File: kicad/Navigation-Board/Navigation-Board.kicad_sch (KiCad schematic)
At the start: 179 parts, among them J25 2.8" TFT, J26 0.96" OLED, J27 Conn_01x02, J28 GME0831B, J31 Conn_01x04, SW10 SW_SPST, SW11 SW_SPST, SW12 SW_SPST, SW13 SW_SPST, SW14 SW_SPST, SW15 SW_SPST, SW16 SW_SPST, SW17 SW_SPST, SW18 SW_SPST, SW19 SW_SPST, SW2 SW_SPST, SW20 SW_SPST, SW21 SW_SPST, SW22 SW_SPST, SW23 SW_SPST, SW24 SW_SPST, SW25 SW_SPST, SW26 SW_SPST, SW27 SW_SPST, SW28 SW_SPST, SW29 SW_SPST, SW3 SW_SPST, SW30 SW_SPST, SW31 SW_SPST, SW32 SW_SPST, SW33 SW_SPST, SW34 SW_SPST, SW35 SW_SPST, SW36 SW_SPST, SW37 SW_SPST, SW38 SW_SPST, SW39 SW_SPST, SW4 SW_SPST, SW40 SW_SPST, SW41 SW_SPST, SW42 SW_SPST, SW43 SW_SPST, SW44 SW_SPST, SW45 SW_SPST, SW46 SW_SPST, SW47 SW_SPST, SW48 SW_SPST, SW49 SW_SPST, SW5 SW_SPST, SW50 SW_SPST, SW51 SW_SPST, SW52 SW_SPST, SW53 SW_SPST, SW54 SW_SPST, SW55 SW_SPST, SW56 SW_SPST, SW57 SW_SPST, SW58 SW_SPST, SW59 SW_SPST, SW6 SW_SPST, SW60 SW_SPST, SW61 SW_SPST, SW62 SW_SPST, SW63 SW_SPST, SW64 SW_SPST, SW65 SW_SPST, SW66 SW_SPST, SW67 SW_SPST, SW68 SW_SPST, SW69 SW_SPST, SW7 SW_SPST, SW70 SW_SPST, SW71 SW_SPST, SW72 SW_SPST, SW73 SW_SPST, SW74 SW_SPST, SW75 SW_SPST, SW76 SW_SPST, SW77 SW_SPST, SW78 SW_SPST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

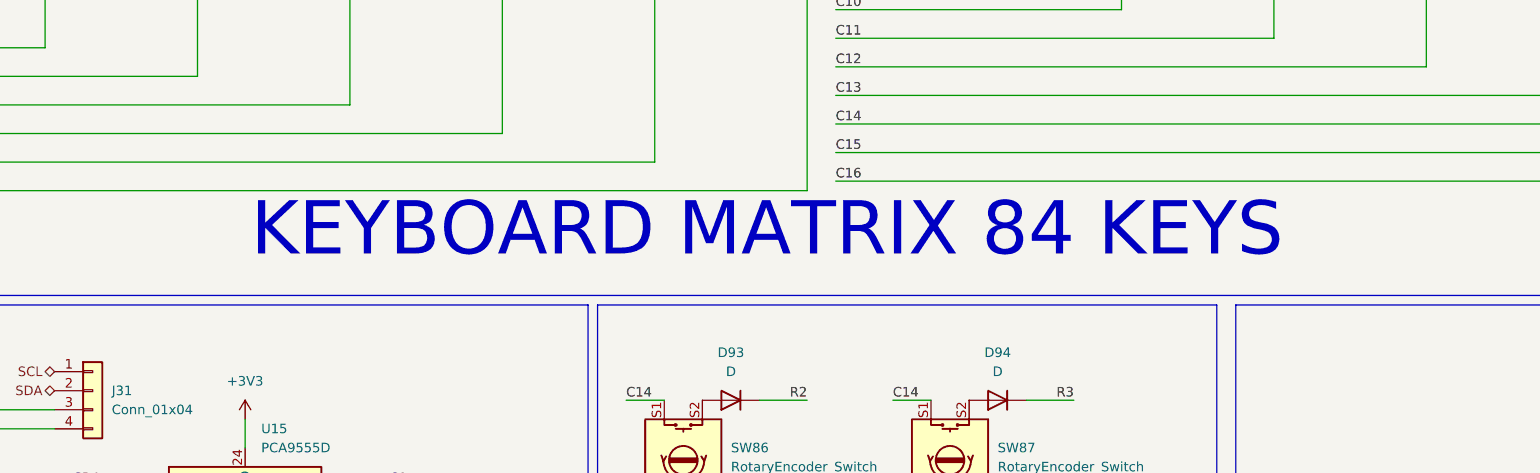
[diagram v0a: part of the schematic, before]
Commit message: upddate
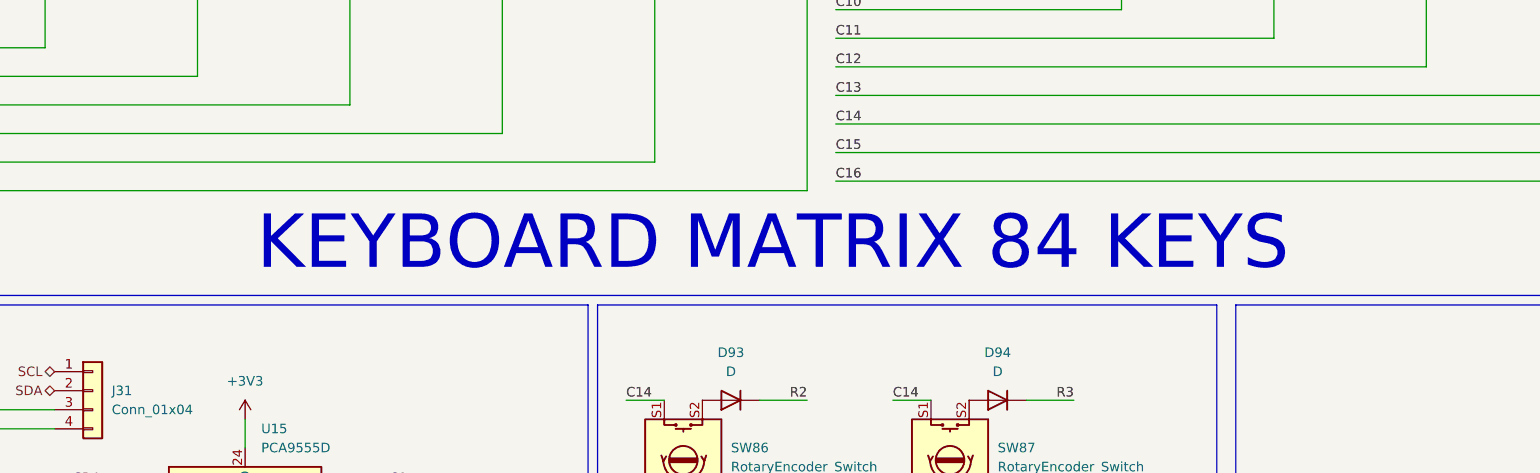
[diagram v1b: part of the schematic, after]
